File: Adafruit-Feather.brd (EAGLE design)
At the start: 58.9 x 45.4 mm, 36 parts, among them Q1 mmbt2222, Q2 mmbt2222, Q3 DMG3415U, SW2 KMR2, U2 AP2112-3.3, U3 MCP73831T-2ACI/OT, X1 JSTPH, X2 ESP32_WROOM32_SKINNY, X4 20329

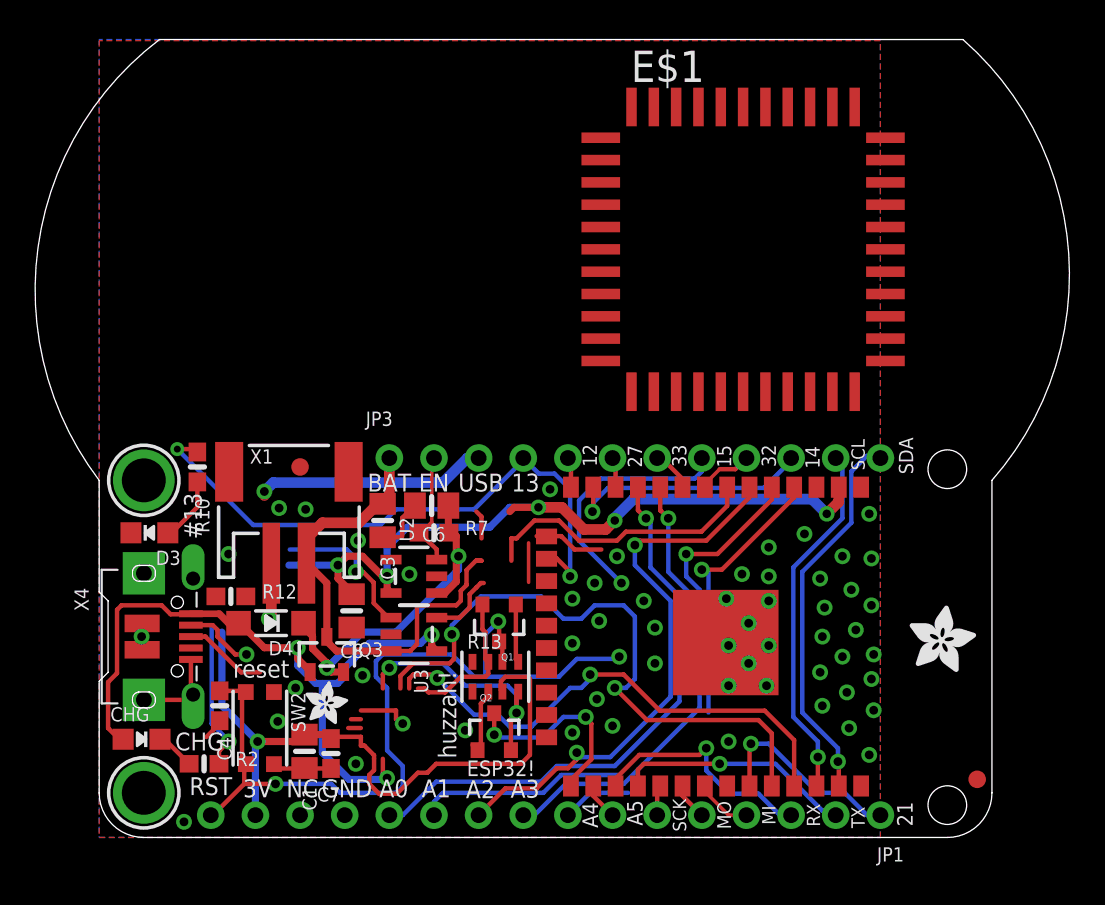
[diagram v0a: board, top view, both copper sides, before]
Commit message: changes
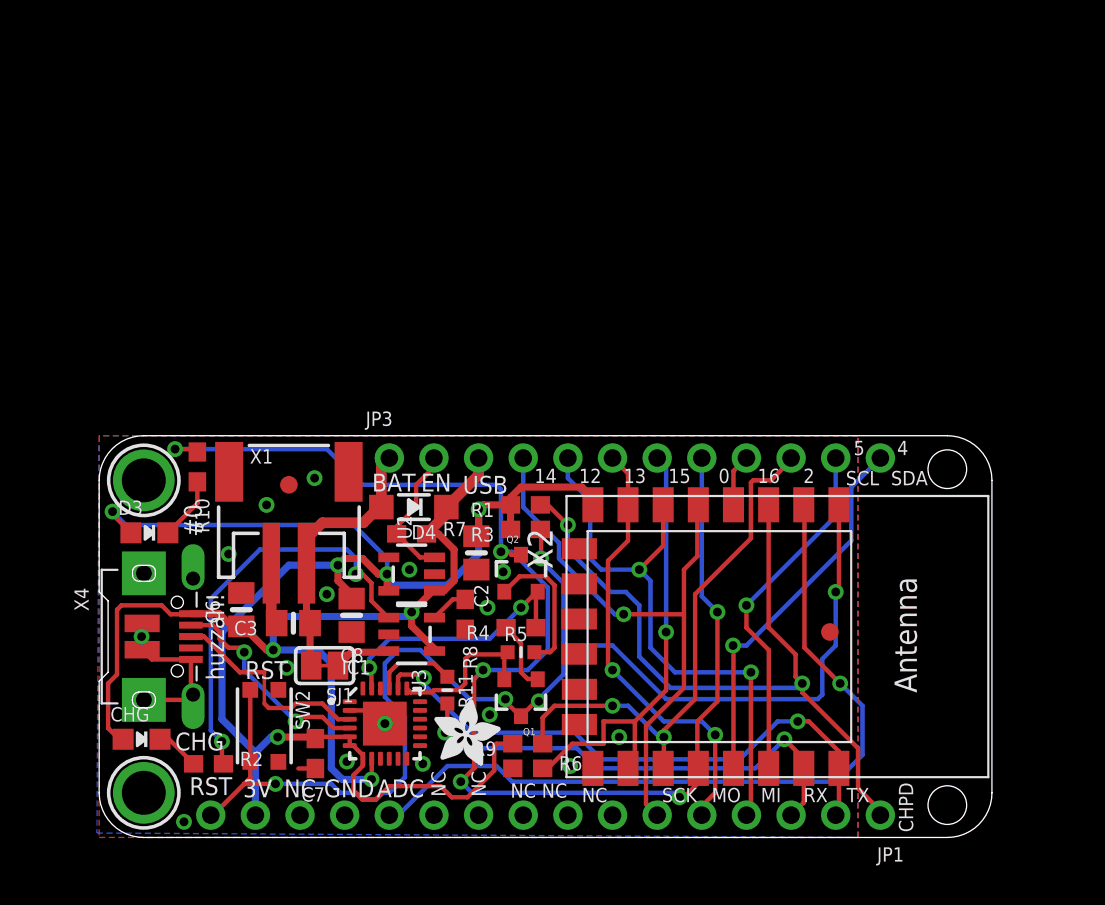
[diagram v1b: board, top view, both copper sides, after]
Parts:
- removed C1: 10uF, microbuilder:0805-NO
- removed C4: 1uF, microbuilder:0603-NO
- removed E$1: (no value), allegro:PLCC44
- removed Q3: DMG3415U, microbuilder:SOT23-R
- removed R12: 100K, microbuilder:0603-NO
- removed R13: 10K, microbuilder:RESPACK_4X0603
- removed U$14: (no value), microbuilder:ADAFRUIT_2.5MM
- removed U$43: (no value), silks:HUZZAH32
- added C2: 10uF, microbuilder:0805-NO
- added IC1: CP2104, microbuilder:QFN24_4MM_SMSC
- added R1, R3, R4, R9: 10K, microbuilder:0603-NO
- added R11: 1K, microbuilder:_0603MP
- added R5: 10K, microbuilder:_0603MP
- added R6: 4.7K, microbuilder:0603-NO
- added R8: 10K\, microbuilder:0603-NO
- added SJ1: (no value), microbuilder:SOLDERJUMPER_CLOSEDWIRE
- added U$23: (no value), microbuilder:HUZZAHLOGO
- JP1: device microbuilder:1X16_ROUND_MIN -> microbuilder:1X16_ROUND
- JP3: device microbuilder:1X12_ROUND_MIN -> microbuilder:1X12_ROUND
- R7: value 100K -> 10K
- U$34, U$35: value FIDUCIAL_1MM -> FIDUCIAL""
- U$9: device silks:FEATHERLOGO_MED -> microbuilder:FEATHERLOGO
- U2: value AP2112-3.3 -> SPX3819
- X2: value ESP32_WROOM32_SKINNY -> ESP-12; device microbuilder:WROOM32_SKINNY -> microbuilder:ESP-12E
- moved U$15 27.6 mm to (19.1, 4.06)
- moved C6 12.3 mm to (8.09, 13.0), turned to 90 degrees
- moved U$35 11.9 mm to (41.6, 11.7)
- moved D4 10.5 mm to (17.9, 18.8)
- moved Q2 9.14 mm to (24.0, 15.0)
- moved C3 7.74 mm to (11.0, 12.2), turned to 180 degrees
- moved U$9 7.04 mm to (30.7, 4.89)
- moved Q1 4.43 mm to (24.0, 8.00)
- moved X2 2.03 mm to (36.3, 11.4)
- moved R7 1.27 mm to (17.8, 17.3)
- moved U$34 1.20 mm to (10.8, 20.1)
- moved U$7 0.90 mm to (45.7, 13.9)
- moved C7 0.89 mm to (12.3, 4.78)
- moved SW2 0.28 mm to (9.40, 6.35)
- moved C8 0.25 mm to (14.4, 12.6)
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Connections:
- removed net A0_DAC2: JP1.12, X2.11
- removed net A13_I35: X2.7
- removed net A1_DAC1: JP1.11
- removed net A2_I34: JP1.10, X2.6
- removed net A3_I39: JP1.9, X2.5
- removed net A4_IO36: JP1.8, X2.4
- removed net A5_IO4: JP1.7, X2.26
- removed net IO12_A11: JP3.5, X2.14
- removed net IO13_A12: JP3.4, R10.1, X2.16
- removed net IO14_A6: JP3.10, X2.13
- removed net IO15_A8: JP3.8, X2.23
- removed net IO16: JP1.3, X2.27
- removed net IO17: JP1.2, X2.28
- removed net IO21: JP1.1, X2.33
- removed net IO27_A10: JP3.6, X2.12
- removed net IO32_A7: JP3.9, X2.8
- removed net IO33_A9: JP3.7, X2.9
- removed net MISO: JP1.4, X2.31
- removed net MOSI: JP1.5, X2.30
- removed net RXD0: X2.34
- removed net S$1: X2.10
- removed net SCK: JP1.6, X2.29
- removed net SCL: JP3.11, X2.36
- removed net SDA: JP3.12, X2.37
- removed net TXD0: X2.35
- new net ADC: JP1.12, X2.2
- new net CH_PD: JP1.1, R1.1, X2.3
- new net GPIO12/MISO: JP1.4, JP3.5, X2.6
- new net GPIO13/MOSI: JP1.5, JP3.6, X2.7
- new net GPIO14/SCK: JP1.6, JP3.4, X2.5
- new net GPIO15: JP3.7, R6.2, X2.10
- new net GPIO16: JP3.9, X2.4
- new net GPIO4/SDA: JP3.12, X2.13
- new net GPIO5/SCL: JP3.11, X2.14
- new net RXD: JP1.3, R11.2, X2.15
- new net TXD: IC1.20, JP1.2, X2.16
- new net USB_RX: IC1.21, R11.1
- net 3.3V: now also C2.1, D3.A, IC1.5, IC1.6, IC1.7, R1.2, R3.2, R9.2, X2.8; no longer C1.1, R13.3, X2.2
- net DTR: now also IC1.23, R4.1; no longer R13.4
- net GND: now also C2.2, IC1.2, IC1.THERM, R6.1, R8.2, X2.9; no longer C1.2, C4.2, D3.C, R12.1, X2.1, X2.15, X2.38, X2.P$1
- net GPIO0: now also JP3.8, R10.1, X2.12; no longer X2.25
- net GPIO2: now also JP3.10, R9.1, X2.11; no longer X2.24
- net N$12: now also R4.2; no longer R13.5
- net N$13: now also R5.2; no longer R13.2
- net N$2: now also IC1.3
- net N$4: now also R8.1
- net N$5: now also D3.C; no longer D3.A
- net N$6: now also IC1.4
- net N$7: now also SJ1.1, U3.3; no longer C6.1, D4.C, Q3.2, R7.2, U2.1
- net RESET: now also R3.1, X2.1; no longer C4.1, R13.6, X2.3
- net RTS: now also IC1.19, R5.1; no longer R13.7
- net VBAT: now also D4.A, SJ1.2; no longer Q3.3, U3.3
- net VBUS: now also C6.1, D4.C, IC1.8, R7.2, U2.1; no longer D4.A, Q3.1, R12.2
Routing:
- net GPIO0: track 11.5 -> 77.7 mm, vias 2 -> 6
- net ADC: track 0.00 -> 44.7 mm, vias 0 -> 1
- net CH_PD: track 0.00 -> 42.4 mm, vias 0 -> 2
- net RXD0: track 36.4 -> 0.00 mm, vias 2 -> 0
- net IO13_A12: track 34.8 -> 0.00 mm, vias 2 -> 0
- net GPIO14/SCK: track 0.00 -> 34.1 mm, vias 0 -> 1
- net TXD: track 0.00 -> 33.3 mm, vias 0 -> 2
- net GPIO12/MISO: track 0.00 -> 32.8 mm, vias 0 -> 2
- net A0_DAC2: track 32.4 -> 0.00 mm, vias 1 -> 0
- net A2_I34: track 31.8 -> 0.00 mm, vias 2 -> 0
- net GPIO2: track 0.00 -> 30.7 mm, vias 0 -> 2
- net TXD0: track 29.3 -> 0.00 mm, vias 2 -> 0
- net A3_I39: track 28.8 -> 0.00 mm, vias 1 -> 0
- net RXD: track 0.00 -> 27.6 mm, vias 0 -> 2
- net RESET: track 48.1 -> 74.4 mm, vias 3 -> 5
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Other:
- board size 58.9 x 45.4 mm -> 50.8 x 22.9 mm
- board text added: "#0"
- board text added: "0"
- board text added: "12/MISO"
- board text added: "13/MOSI"
- board text added: "14/SCK"
- board text added: "16"
- board text added: "2"
- board text added: "4"
- board text added: "4MB Flash 80MHz & 3.3V"
- board text added: "5"
- board text added: "ADC"
- board text added: "CHPD"
- board text added: "Feather HUZZAH ESP8266 WiFi"
- board text added: "SCL/5"
- board text added: "SDA/4"
- board text removed: "#13"
- board text removed: "12/A11"
- board text removed: "13/A12"
- board text removed: "14/A6"
- board text removed: "15/A8"
- board text removed: "21"
- board text removed: "27"
- board text removed: "27/A10"
- board text removed: "32"
- board text removed: "32/A7"
- board text removed: "33"
- board text removed: "33/A9"
- board text removed: "A0"
- board text removed: "A0 DAC2"
- board text removed: "A1"
- board text removed: "A1 DAC1"
- board text removed: "A2"
- board text removed: "A2/34"
- board text removed: "A3"
- board text removed: "A3/39"
- board text removed: "A4"
- board text removed: "A4/36"
- board text removed: "A5"
- board text removed: "A5/4"
- board text removed: "Contains FCCID 2AC7Z-ESP32"
- board text removed: "ESP32 Feather 16MB Flash WiFI+BT"
- board text removed: "ESP32!"
- board text removed: "MISO/19"
- board text removed: "MOSI/18"
- board text removed: "RX/16"
- board text removed: "SCK/5"
- board text removed: "SCL/22"
- board text removed: "SDA/23"
- board text removed: "TX/17"
- board text removed: "reset"
